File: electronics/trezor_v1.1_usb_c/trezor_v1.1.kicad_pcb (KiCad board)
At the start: 2 copper layers, 50 x 26.7 mm, 34 parts, among them IC1 MCP1703T-3302E/CB, J1 USB_C_Receptacle_USB2.0, K2 SWD, Q2 8MHz, U1 STM32F205RET6, U3 DISPLAY

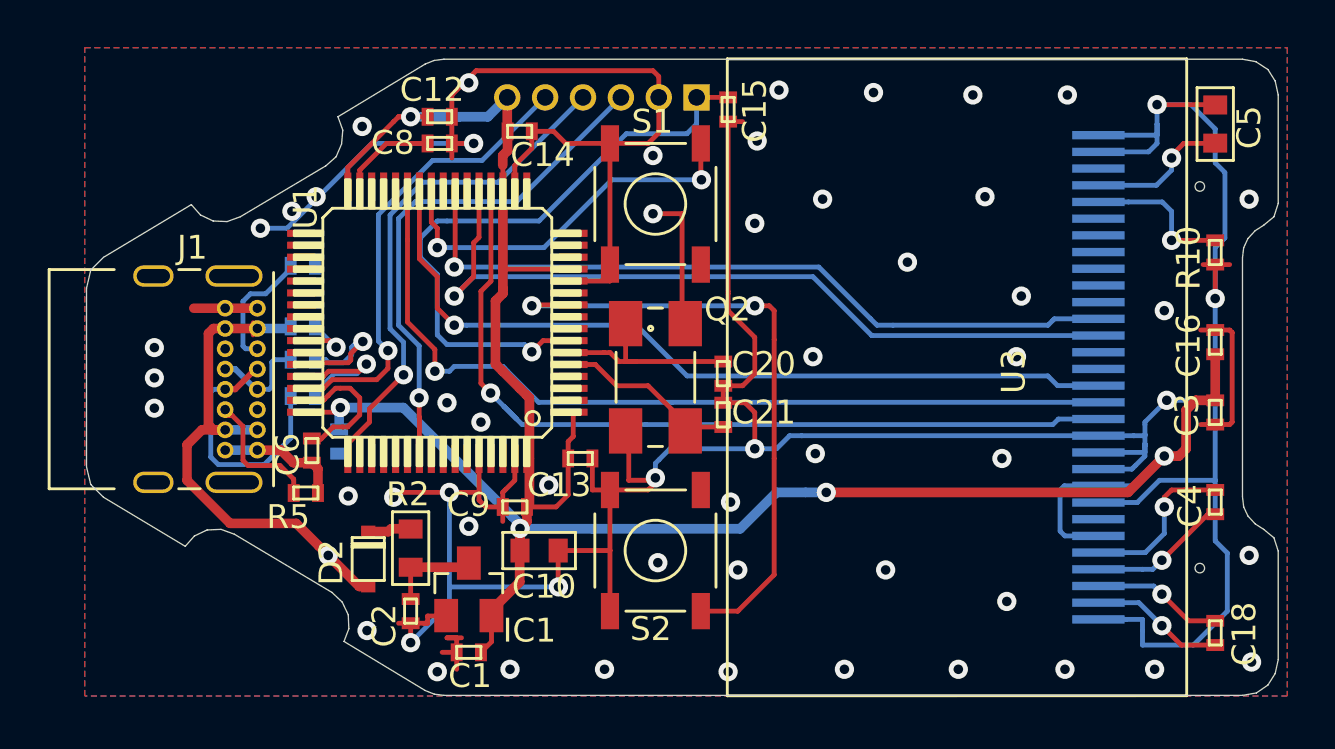
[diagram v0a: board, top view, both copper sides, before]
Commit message: Fix solder mask on all footprints, minor trace cleanup
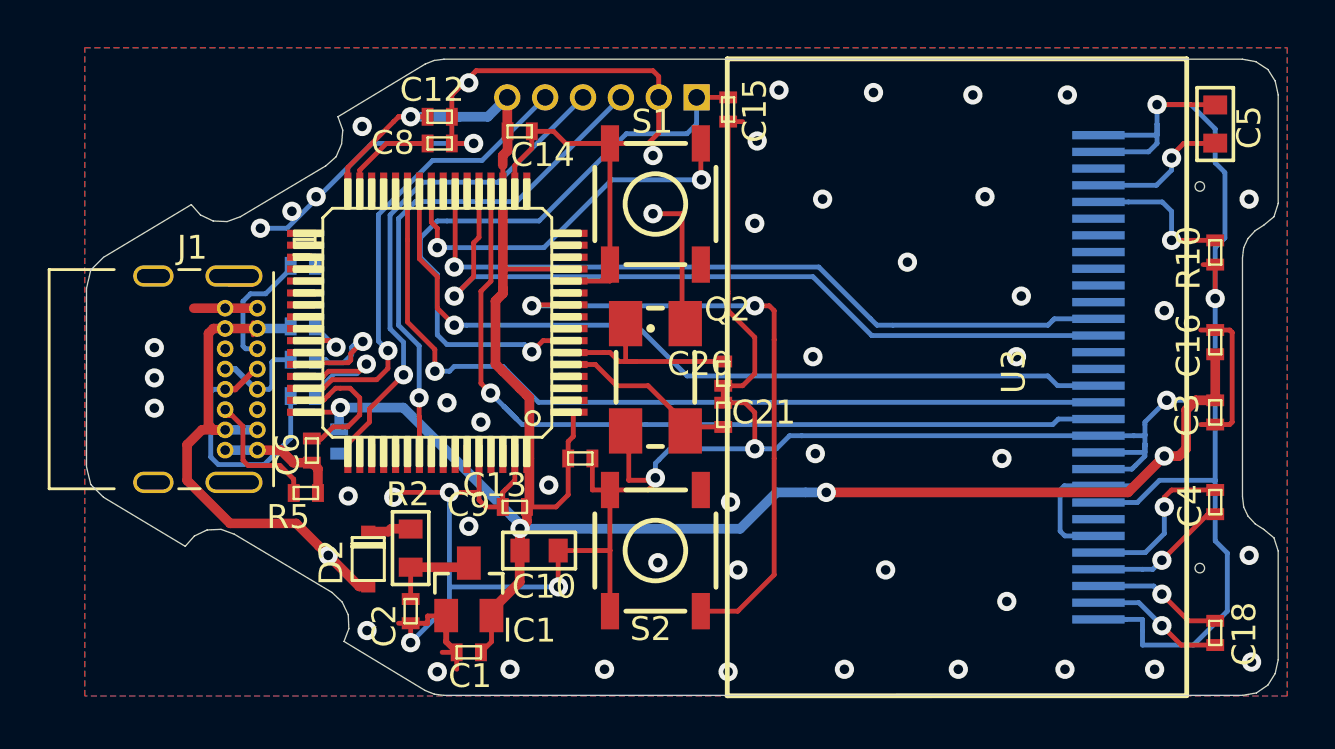
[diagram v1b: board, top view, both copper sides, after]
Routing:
- net GND: track 200.9 -> 199.0 mm
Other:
- rule pad_to_mask_clearance: 0.051 -> 0.05
- rule solder_mask_min_width: 0.25 -> 0.05
